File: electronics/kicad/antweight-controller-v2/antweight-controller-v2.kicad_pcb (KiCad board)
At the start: 2 copper layers, 30.5 x 58.4 mm, 11 parts, among them J10 3V3 GND VBAT_SW, J4 BATTERY, J5 MOTOR LEFT, J6 MOTOR RIGHT, J8 ESP32 LEFT ALL PINS, J9 ESP32 RIGHT SIGNALS, SW1 MAIN POWER, U1 ESP32-C3 SUPERMINI, U2 DRV8833, U3 3V3 BUCK-BOOST

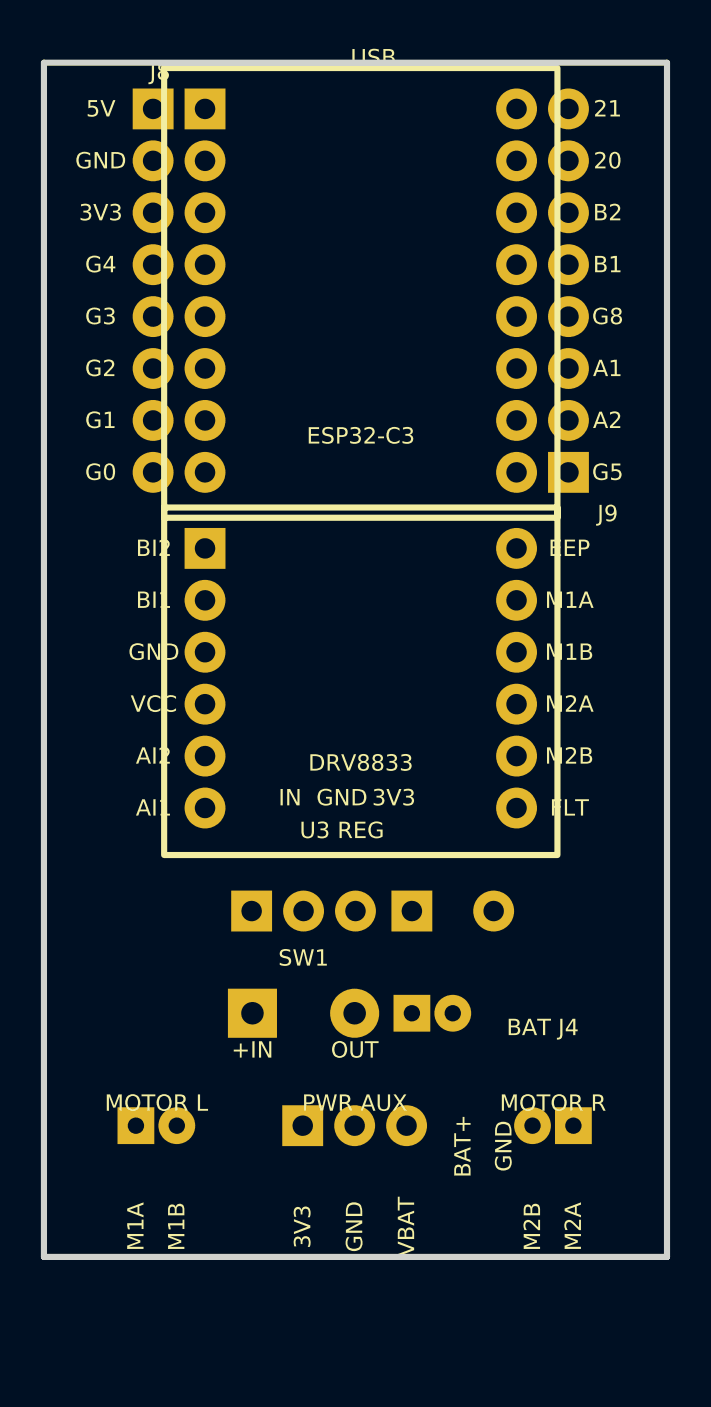
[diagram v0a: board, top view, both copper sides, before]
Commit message: feat(electronics): finalize v2 controller layout
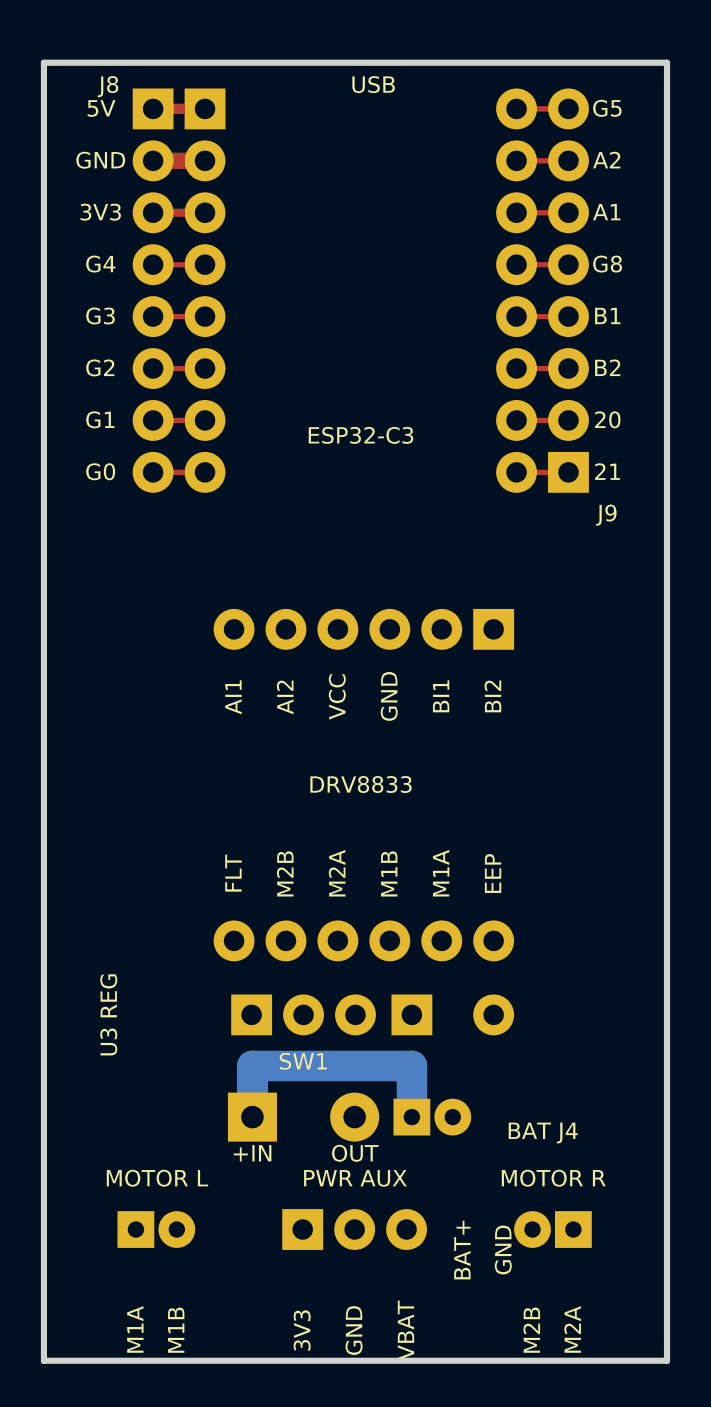
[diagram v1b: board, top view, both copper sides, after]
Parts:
- moved U2 14.7 mm to (22.0, 27.7), turned to 270 degrees
- moved C1_C2 5.08 mm to (18.0, 46.6)
- moved J10 5.08 mm to (12.7, 57.1)
- moved J4 5.08 mm to (18.0, 51.6)
- moved J5 5.08 mm to (4.50, 57.1)
- moved J6 5.08 mm to (25.9, 57.1)
- moved SW1 5.08 mm to (10.2, 51.6)
- moved U3 5.08 mm to (10.2, 46.6)
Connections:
- J9 pad 1: GPIO5_SPARE -> GPIO21_SPARE
- J9 pad 2: AIN2_GPIO6 -> GPIO20_SPARE
- J9 pad 3: AIN1_GPIO7 -> BIN2_GPIO10
- J9 pad 4: GPIO8_LED_EXPANSION -> BIN1_GPIO9
- J9 pad 5: BIN1_GPIO9 -> GPIO8_LED_EXPANSION
- J9 pad 6: BIN2_GPIO10 -> AIN1_GPIO7
- J9 pad 7: GPIO20_SPARE -> AIN2_GPIO6
- J9 pad 8: GPIO21_SPARE -> GPIO5_SPARE
- U1 pad 10: AIN2_GPIO6 -> GPIO20_SPARE
- U1 pad 11: AIN1_GPIO7 -> BIN2_GPIO10
- U1 pad 12: GPIO8_LED_EXPANSION -> BIN1_GPIO9
- U1 pad 13: BIN1_GPIO9 -> GPIO8_LED_EXPANSION
- U1 pad 14: BIN2_GPIO10 -> AIN1_GPIO7
- U1 pad 15: GPIO20_SPARE -> AIN2_GPIO6
- U1 pad 16: GPIO21_SPARE -> GPIO5_SPARE
- U1 pad 9: GPIO5_SPARE -> GPIO21_SPARE
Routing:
- net VBAT_RAW: track 0.00 -> 12.8 mm
- net GPIO4_SPARE: track 0.00 -> 2.54 mm
- net GPIO3_SPARE: track 0.00 -> 2.54 mm
- net GPIO2_SPARE: track 0.00 -> 2.54 mm
- net GPIO1_SPARE: track 0.00 -> 2.54 mm
- net GPIO0_SPARE: track 0.00 -> 2.54 mm
- net GND: track 0.00 -> 2.54 mm
- net 5V_NC: track 0.00 -> 2.54 mm
- net 3V3: track 0.00 -> 2.54 mm
- net GPIO8_LED_EXPANSION: track 0.00 -> 2.54 mm
- net GPIO5_SPARE: track 0.00 -> 2.54 mm
- net GPIO21_SPARE: track 0.00 -> 2.54 mm
- net GPIO20_SPARE: track 0.00 -> 2.54 mm
- net BIN2_GPIO10: track 0.00 -> 2.54 mm
- net BIN1_GPIO9: track 0.00 -> 2.54 mm
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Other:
- board size 30.5 x 58.4 mm -> 30.5 x 63.5 mm
- board text removed: "IN"
